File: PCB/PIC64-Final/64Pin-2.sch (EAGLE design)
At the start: 159 parts, among them IC1 , IC2 , IC3 , IC4 , J1 84952-4, Q1 , X2 , X3 , X4 , X5 , X6 , X7 , X8 , X9 

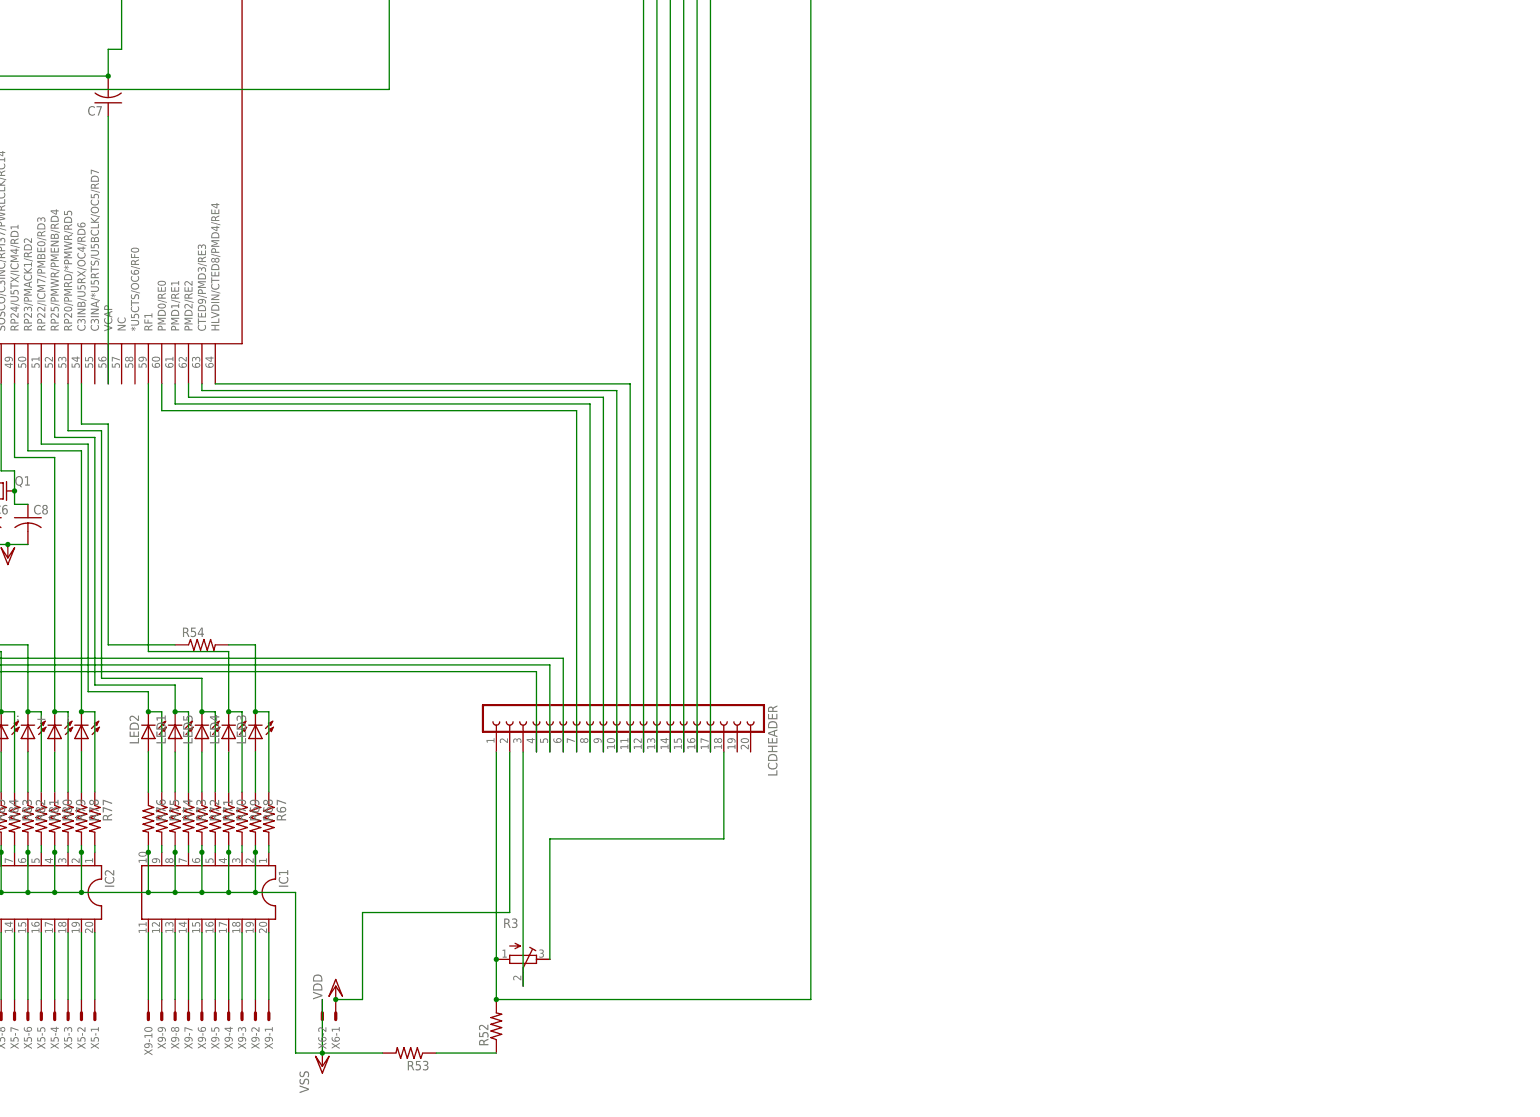
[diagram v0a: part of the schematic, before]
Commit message: nd
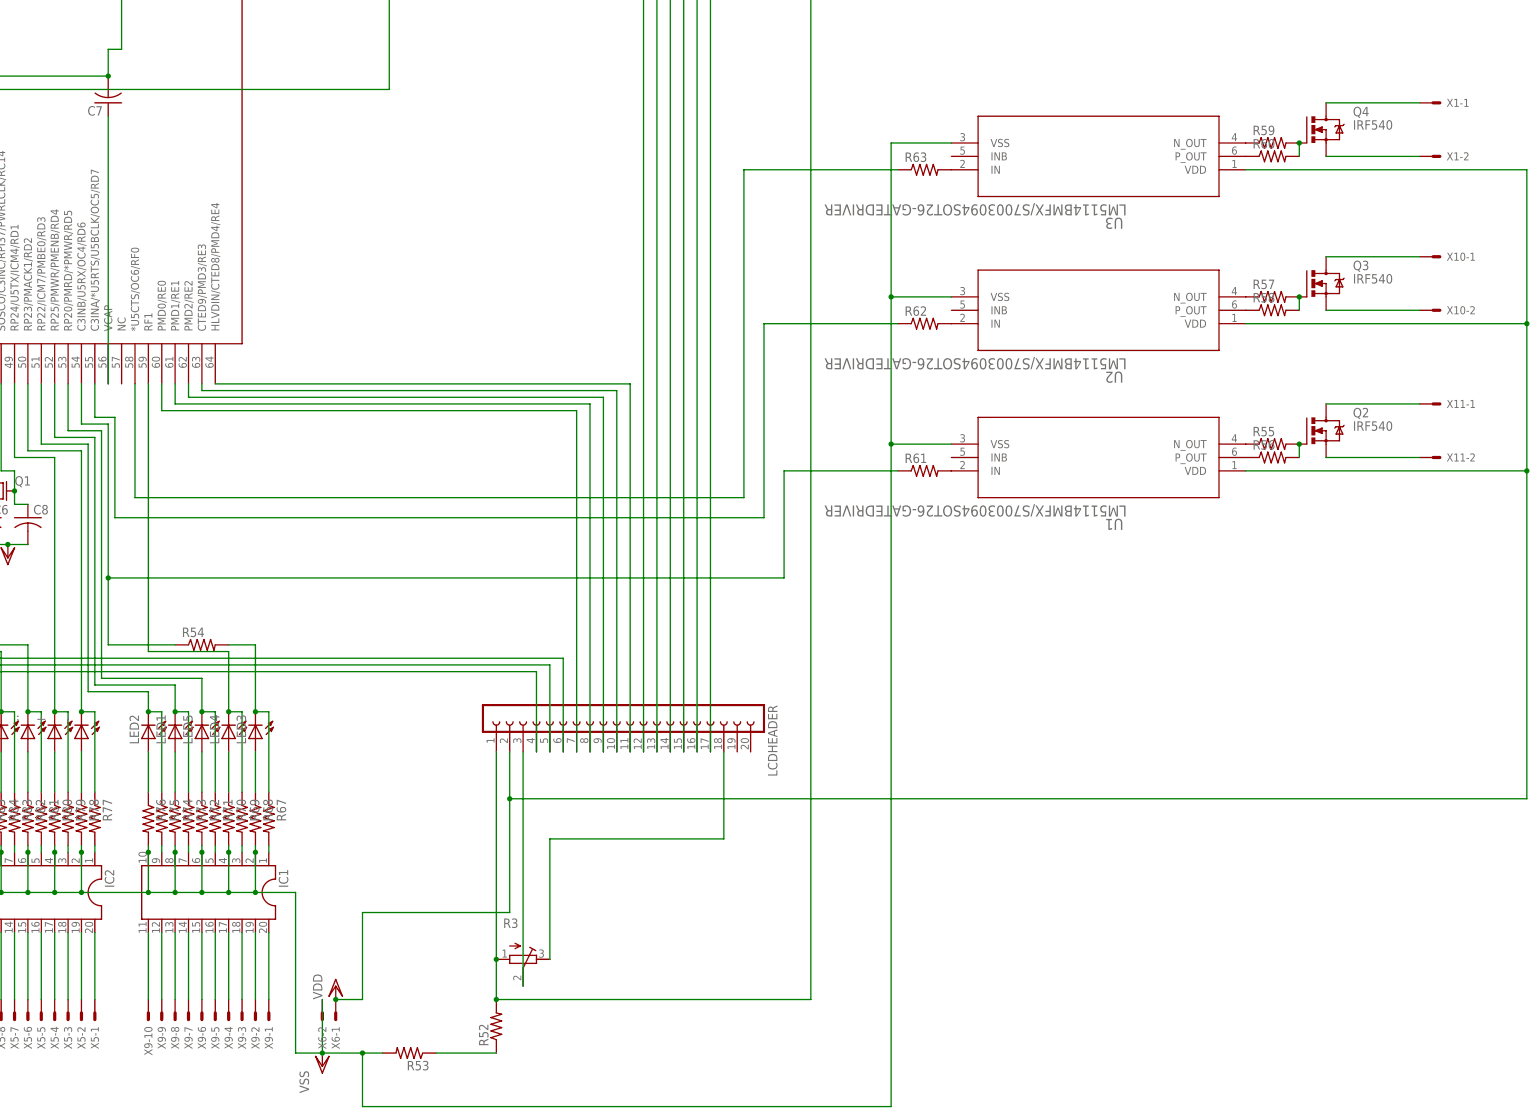
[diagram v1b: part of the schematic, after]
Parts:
- added Q2, Q3, Q4: IRF540, transistor-power:IRF540
- added R55, R56, R57, R58, R59, R60, R61, R62, R63: (no value), resistor:R-US_R0603
- added U1, U2, U3: LM5114BMFX/S7003094SOT26-GATEDRIVER, SOT26:LM5114BMFX/S7003094SOT26-GATEDRIVER
- added X1, X10, X11: (no value), con-molex:KK-156-2
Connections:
- new net N$33: R57.1, U2.N_OUT
- new net N$34: R58.1, U2.P_OUT
- new net N$35: R55.1, U1.N_OUT
- new net N$41: R56.1, U1.P_OUT
- new net N$48: Q2.G, R55.2, R56.2
- new net N$50: Q3.G, R57.2, R58.2
- new net N$52: R59.1, U3.N_OUT
- new net N$59: R60.1, U3.P_OUT
- new net N$61: Q4.G, R59.2, R60.2
- new net N$63: Q4.D, X1-1.S
- new net N$65: Q4.S, X1-2.S
- new net N$67: Q3.D, X10-1.S
- new net N$74: Q3.S, X10-2.S
- new net N$75: Q2.D, X11-1.S
- new net N$76: Q2.S, X11-2.S
- new net N$77: R61.2, U1.IN
- new net N$78: R62.2, U2.IN
- new net N$79: R63.2, U3.IN
- new net N$80: P.C3INA/*U5RTS/U5BCLK/OC5/RD7, R62.1
- new net N$81: P.*U5CTS/OC6/RF0, R63.1
- net PIN54: now also R61.1
- net VDD: now also U1.VDD, U2.VDD, U3.VDD
- net VSS: now also U1.VSS, U2.VSS, U3.VSS
